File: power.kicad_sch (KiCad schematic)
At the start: 15 parts, among them J1 GT-USB-7010ASV, P1 S2B-PH-SM4-TB, U1 BQ25185DLHR, U2 TPS73633DBVT

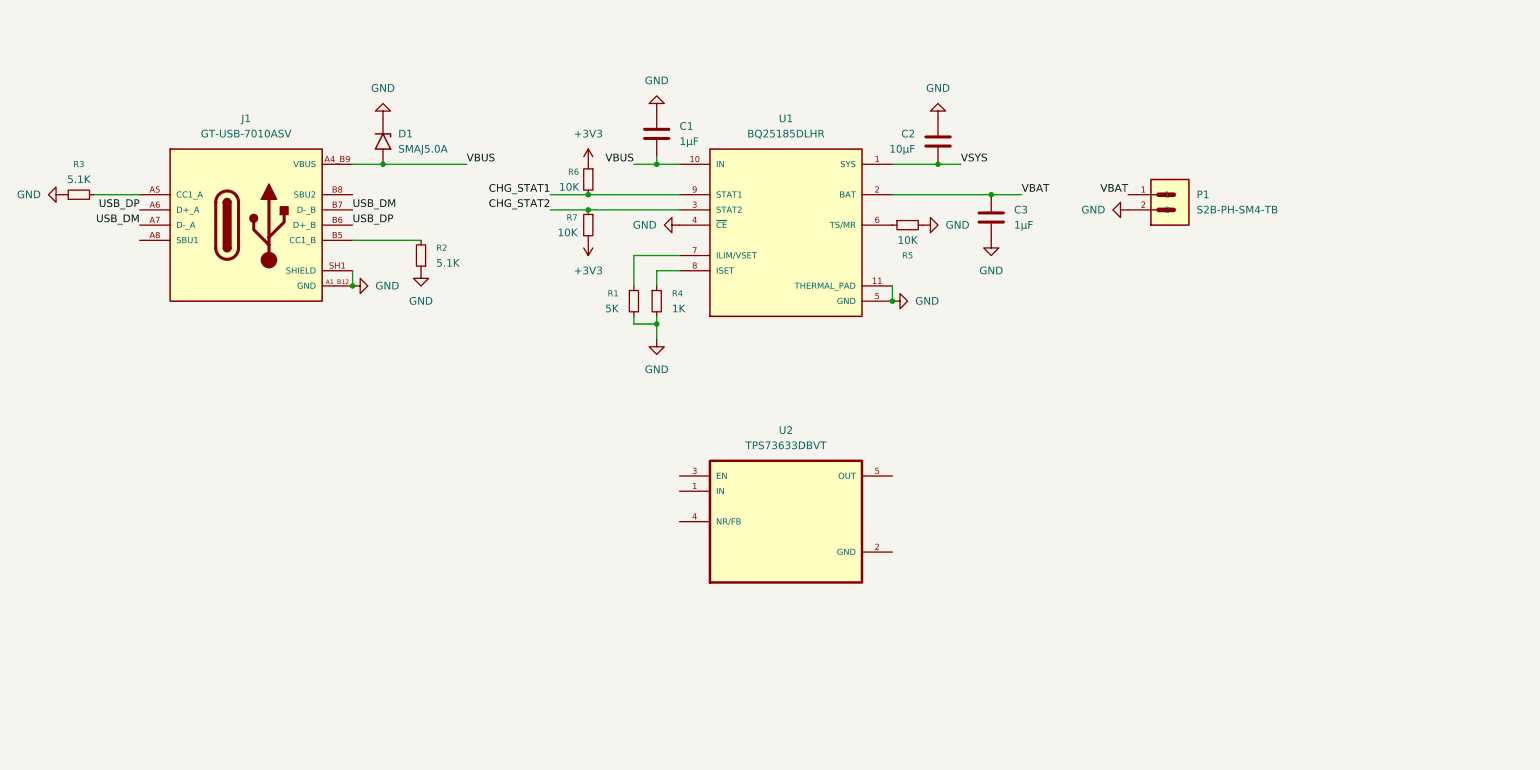
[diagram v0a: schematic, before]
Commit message: finish power schematic
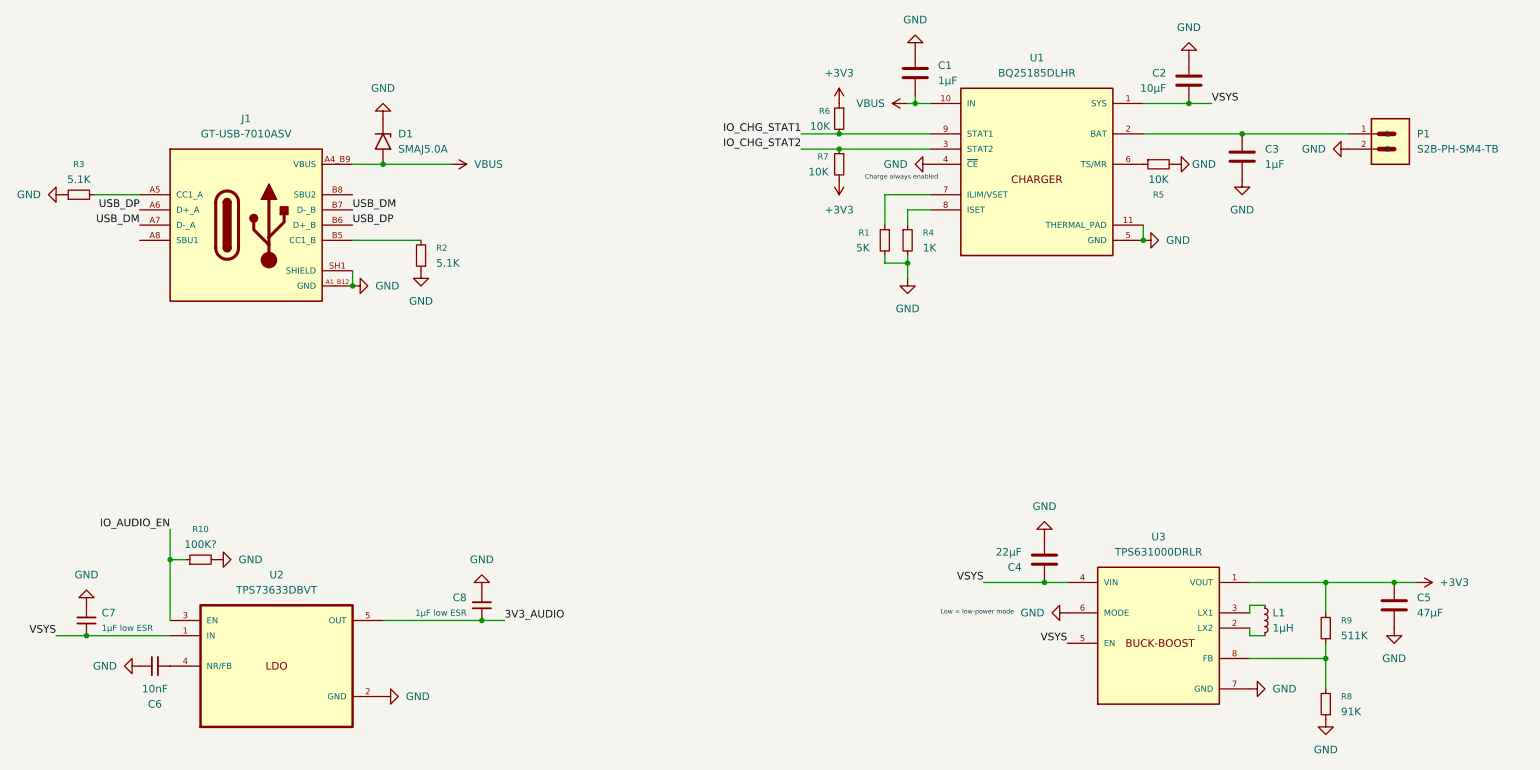
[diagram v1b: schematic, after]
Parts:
- added C4: 22µF, Package_DFN_QFN:VQFN-16-1EP_3x3mm_P0.5mm_EP1.6x1.6mm, symbol Device:C
- added C5: 47µF, Package_DFN_QFN:VQFN-16-1EP_3x3mm_P0.5mm_EP1.6x1.6mm, symbol Device:C
- added C6: 10nF, symbol Device:C_Small
- added C7, C8: 1µF low ESR, symbol Device:C_Small
- added L1: 1μH, symbol Device:L_Small
- added R10: 100K?, symbol Device:R_Small
- added R8: 91K, symbol Device:R_Small
- added R9: 511K, symbol Device:R_Small
- added U3: TPS631000DRLR, TPS631000DRLR:SOT50P160X60-8N, symbol TPS631000DRLR:TPS631000DRLR
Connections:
- net +3V3: now also C5.2, R9.2, U3.1 (VOUT)
- net GND: now also U2.2 (GND), C4.1, C5.1, C6.1, C7.1, C8.1, R10.2, R8.1, U3.6 (MODE), U3.7 (GND)
- net VSYS: now also U2.1 (IN), C4.2, C7.2, U3.4 (VIN), U3.5 (EN)
- net IO_AUDIO_EN: now reaches U2.3 (EN)
- net IO_AUDIO_EN: now also R10.1
- net at U2.4 (NR/FB): now also C6.2
- net 3V3_AUDIO: now reaches U2.5 (OUT)
- net 3V3_AUDIO: now also C8.2
- net CHG_STAT1 renamed IO_CHG_STAT1
- net CHG_STAT2 renamed IO_CHG_STAT2
- net VBAT: no longer names the net of C3.2, P1.1, U1.2 (BAT)
- new net: L1.1, U3.3 (LX1)
- new net: L1.2, U3.2 (LX2)
- new net: R8.2, R9.1, U3.8 (FB)
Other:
- note added: "Charge always enabled"
- note added: "Low = low-power mode"
- moved on the sheet: C1, C2, C3, P1, R1, R4, R5, R6, R7
